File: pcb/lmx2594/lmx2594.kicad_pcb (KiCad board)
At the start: 2 copper layers, 48.3 x 48.3 mm, 80 parts, among them J1 Conn_Coaxial, J2 Conn_Coaxial, J3 Conn_01x13_Male, J4 Conn_Coaxial, J5 Conn_Coaxial, J6 Conn_Coaxial, J7 Conn_Coaxial, J8 Conn_Coaxial, J9 Conn_Coaxial, U1 L7812, U2 TPS62150, U3 lmx254

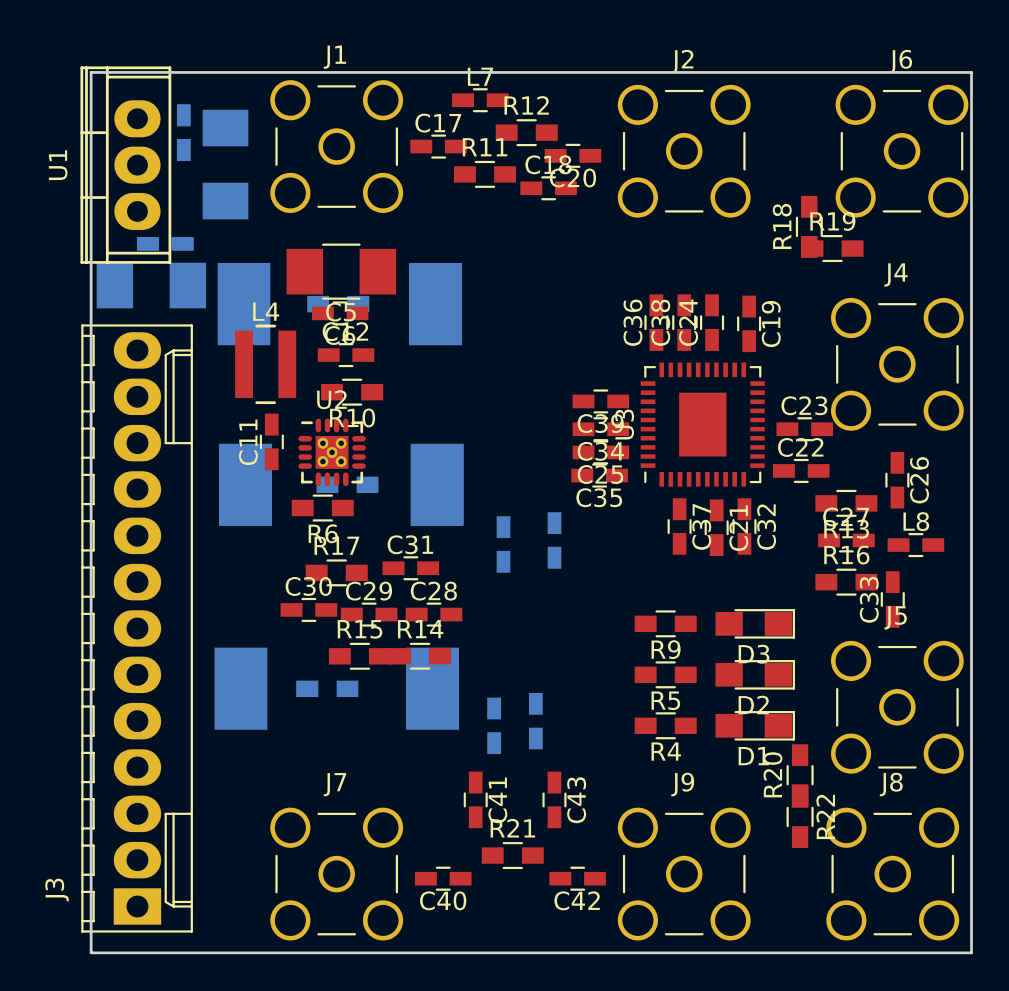
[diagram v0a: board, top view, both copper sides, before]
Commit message: More work on layout
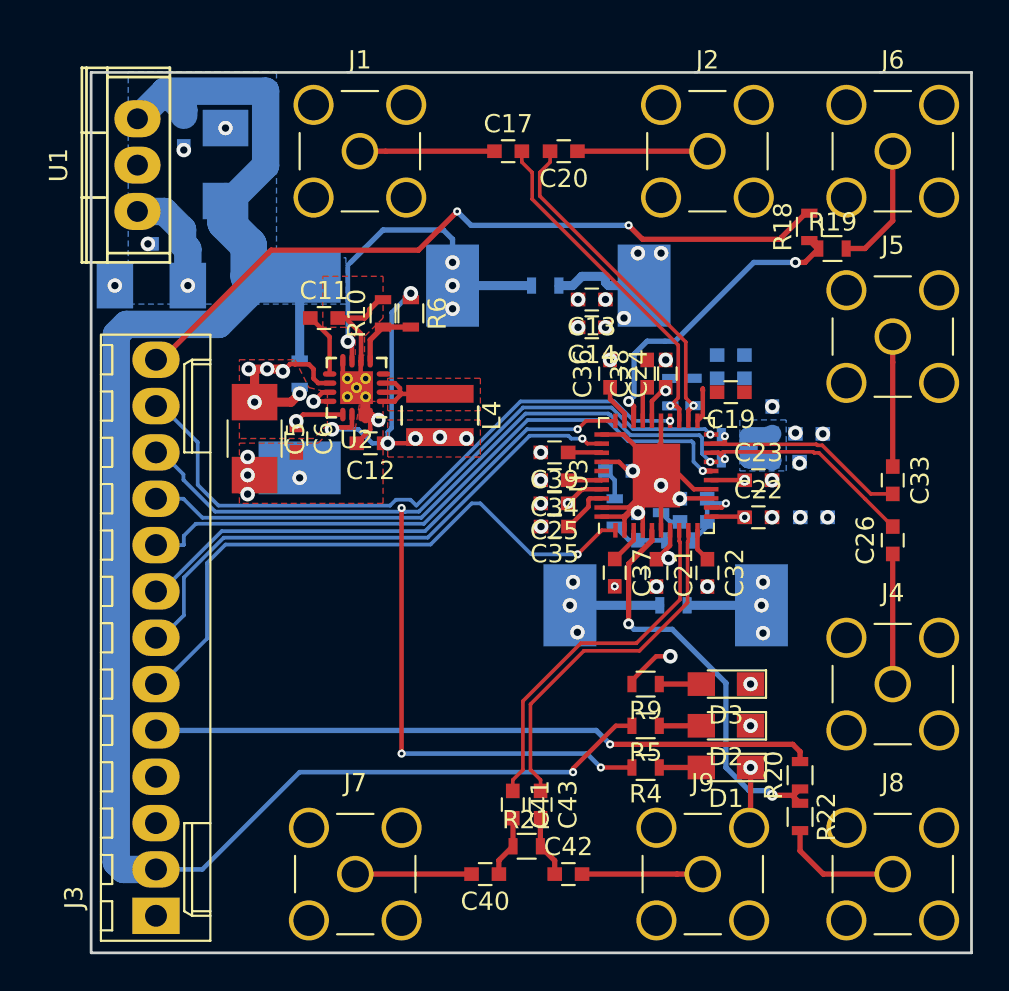
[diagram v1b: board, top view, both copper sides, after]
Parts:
- C11, C12, C17, C19, C2, C20, C21, C22, C23, C24, C25, C26, C3, C32, C33, C34, C35, C36, C37, C38, C39, C40, C41, C42, C43, C6, C7, C8: footprint Capacitors_SMD:C_0603_HandSoldering -> Capacitors_SMD:C_0603
- C13, C14: footprint Capacitors_SMD:C_0603_HandSoldering -> Capacitors_SMD:C_0603; moved to F.Cu
- C18, C27, C28, C29, C30, C31, L7, L8: footprint Capacitors_SMD:C_0603_HandSoldering -> Capacitors_SMD:C_0603; moved to B.Cu
- R1, R10, R18, R19, R2, R20, R21, R22, R4, R5, R6, R7, R9: footprint Resistors_SMD:R_0603_HandSoldering -> Resistors_SMD:R_0603
- R11, R12, R13, R14, R15, R16, R17: footprint Resistors_SMD:R_0603_HandSoldering -> Resistors_SMD:R_0603; moved to B.Cu
- moved R7 25.1 mm to (98.6, 82.8)
- moved L5 25.0 mm to (98.7, 82.8)
- moved C13 24.0 mm to (101.1, 83.6), turned to 180 degrees
- moved C14 21.8 mm to (101.1, 85.1), turned to 180 degrees
- moved C30 21.6 mm to (106.7, 95.8), turned to 180 degrees
- moved J5 20.3 mm to (117.6, 85.6)
- moved L7 19.6 mm to (108.7, 86.6)
- moved R2 19.0 mm to (105.6, 100.3)
- moved L1 19.0 mm to (105.2, 100.3)
- moved R15 18.6 mm to (105.9, 96.8), turned to 180 degrees
- moved R17 18.2 mm to (104.9, 94.5), turned to 270 degrees
- moved J4 17.5 mm to (117.6, 104.6)
- moved C7 17.1 mm to (113.3, 95.5), turned to 0 degrees
- moved R12 16.9 mm to (106.7, 88.6), turned to 270 degrees
- moved C31 16.0 mm to (106.7, 94.5), turned to 180 degrees
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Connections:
- net Net-(C17-Pad2) renamed /RFOUT_A_P
- net Net-(C18-Pad2) renamed /RFA_BIAS
- net Net-(C20-Pad2) renamed /RFOUT_A_N
- net Net-(C26-Pad2) renamed /RFOUT_B_N
- net Net-(C27-Pad2) renamed /RFB_BIAS
- net Net-(C28-Pad1) renamed /VTUNE
- net Net-(C30-Pad1) renamed /CPOUT
- net Net-(C33-Pad2) renamed /RFOUT_B_P
- net Net-(C41-Pad1) renamed /OSCIN_P
- net Net-(C43-Pad1) renamed /OSCIN_N
- net Net-(L4-Pad1) renamed /SW
- C12 pad 1: Net-(C12-Pad1) -> /3V3
- C3 pad 1: Net-(C3-Pad1) -> /12V_unfilt
- C4 pad 1: Net-(C3-Pad1) -> /12V_unfilt
- J3 pad 10: /SYSREFREQ_S -> /SDI
- J3 pad 11: /RAMPCLK -> /MUX
- J3 pad 12: /RAMPDIR -> /CSB
- J3 pad 13: /MUX -> /SYSREF_REQ_S
- J3 pad 2: /12V -> /12V_unfilt
- J3 pad 4: /VCC -> /3V3
- J3 pad 5: /CE -> /SYNC_S
- J3 pad 6: /CSB -> /CE
- J3 pad 7: /SDI -> /RAMPDIR
- J3 pad 8: /SCK -> /RAMPCLK
- J3 pad 9: /SYNC_S -> /SCK
- L1 pad 1: Net-(C12-Pad1) -> /3V3
- L3 pad 1: Net-(C3-Pad1) -> /12V_unfilt
- L4 pad 2: Net-(C12-Pad1) -> /3V3
- L5 pad 1: Net-(C12-Pad1) -> /3V3
- R1 pad 2: Net-(C3-Pad1) -> /12V_unfilt
- R18 pad 1: /SYNC -> /SYSREFREQ
- R18 pad 2: /SYNC_S -> /SYSREF_REQ_S
- R19 pad 1: /SYNC -> /SYSREFREQ
- R2 pad 2: Net-(C12-Pad1) -> /3V3
- R20 pad 1: /SYSREFREQ -> /SYNC
- R20 pad 2: /SYSREF_REQ_S -> /SYNC_S
- R22 pad 1: /SYSREFREQ -> /SYNC
- R5 pad 2: /12V -> /12V_unfilt
- R6 pad 1: Net-(C12-Pad1) -> /3V3
- R7 pad 2: Net-(C12-Pad1) -> /3V3
- U1 pad 3: Net-(C3-Pad1) -> /12V_unfilt
- U2 pad 14: Net-(C12-Pad1) -> /3V3
- U2 pad 7: Net-(C12-Pad1) -> /3V3
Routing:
- net GND: track 0.00 -> 364.4 mm, vias 0 -> 31
- net /12V_unfilt: track 0.00 -> 98.4 mm, vias 0 -> 1
- net /3V3: track 0.00 -> 96.8 mm, vias 0 -> 13
- net /VCC: track 0.00 -> 66.0 mm, vias 0 -> 11
- net /MUX: track 0.00 -> 61.6 mm, vias 0 -> 4
- net /VIN: track 0.00 -> 51.1 mm, vias 0 -> 1
- net /SYSREF_REQ_S: track 0.00 -> 40.5 mm, vias 0 -> 2
- net /SYNC_S: track 0.00 -> 36.3 mm, vias 0 -> 1
- net /SCK: track 0.00 -> 35.3 mm, vias 0 -> 1
- net /CSB: track 0.00 -> 34.9 mm, vias 0 -> 1
- net /SDI: track 0.00 -> 34.8 mm, vias 0 -> 1
- net /CE: track 0.00 -> 33.4 mm, vias 0 -> 1
- net /RAMPDIR: track 0.00 -> 30.4 mm, vias 0 -> 1
- net /RAMPCLK: track 0.00 -> 29.1 mm, vias 0 -> 1
- net /SYNC: track 0.00 -> 22.4 mm, vias 0 -> 2
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- added copper zone on F.Cu, net /12V
- added copper zone on In2.Cu, net /12V
- added copper zone on B.Cu, net /12V_unfilt
- added copper zone on F.Cu, net /3V3
- added copper zone on In2.Cu, net /3V3
- added copper zone on B.Cu, net /RFB_BIAS
- added copper zone on F.Cu, net /SW
- added copper zone on In2.Cu, net /VCC
- added copper zone on In2.Cu, net /VIN
- added copper zone on In2.Cu, net /VRF
- added copper zone on F.Cu, net GND
- added copper zone on In1.Cu, net GND
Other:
- copper layers 2 -> 4
- net class Default: clearance 0.2 -> 0.127; trace_width 0.25 -> 0.0889
- rule trace_clearance: 0.2 -> 0.127
- rule trace_min: 0.2 -> 0.0889
- rule via_min_drill: 0.3 -> 0.2
